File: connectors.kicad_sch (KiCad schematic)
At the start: 17 parts, among them J1 USB_C_Receptacle_USB2.0, J2 Power_Input, J3 Conn_01x11_Socket, J4 MOTOR_1_OUTPUT, J5 MOTOR_2_OUTPUT, J6 MOTOR_3_OUTPUT, J7 MOTOR_4_OUTPUT, J8 Conn_01x03_Socket, J9 Conn_01x11_Socket, U3 USBLC6-2SC6

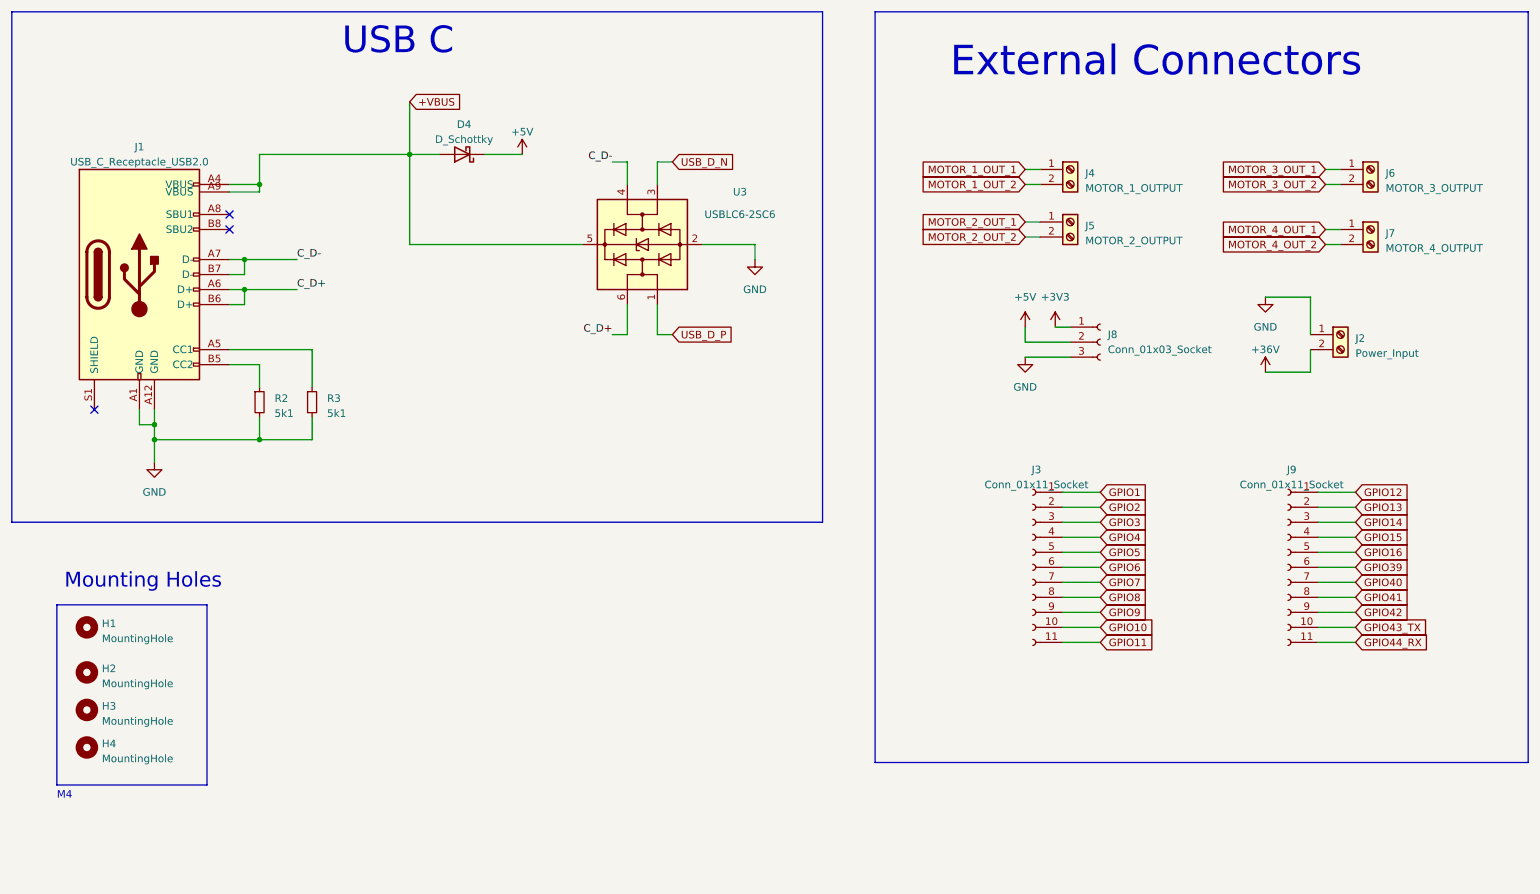
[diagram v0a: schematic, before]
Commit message: checkpoint for backup
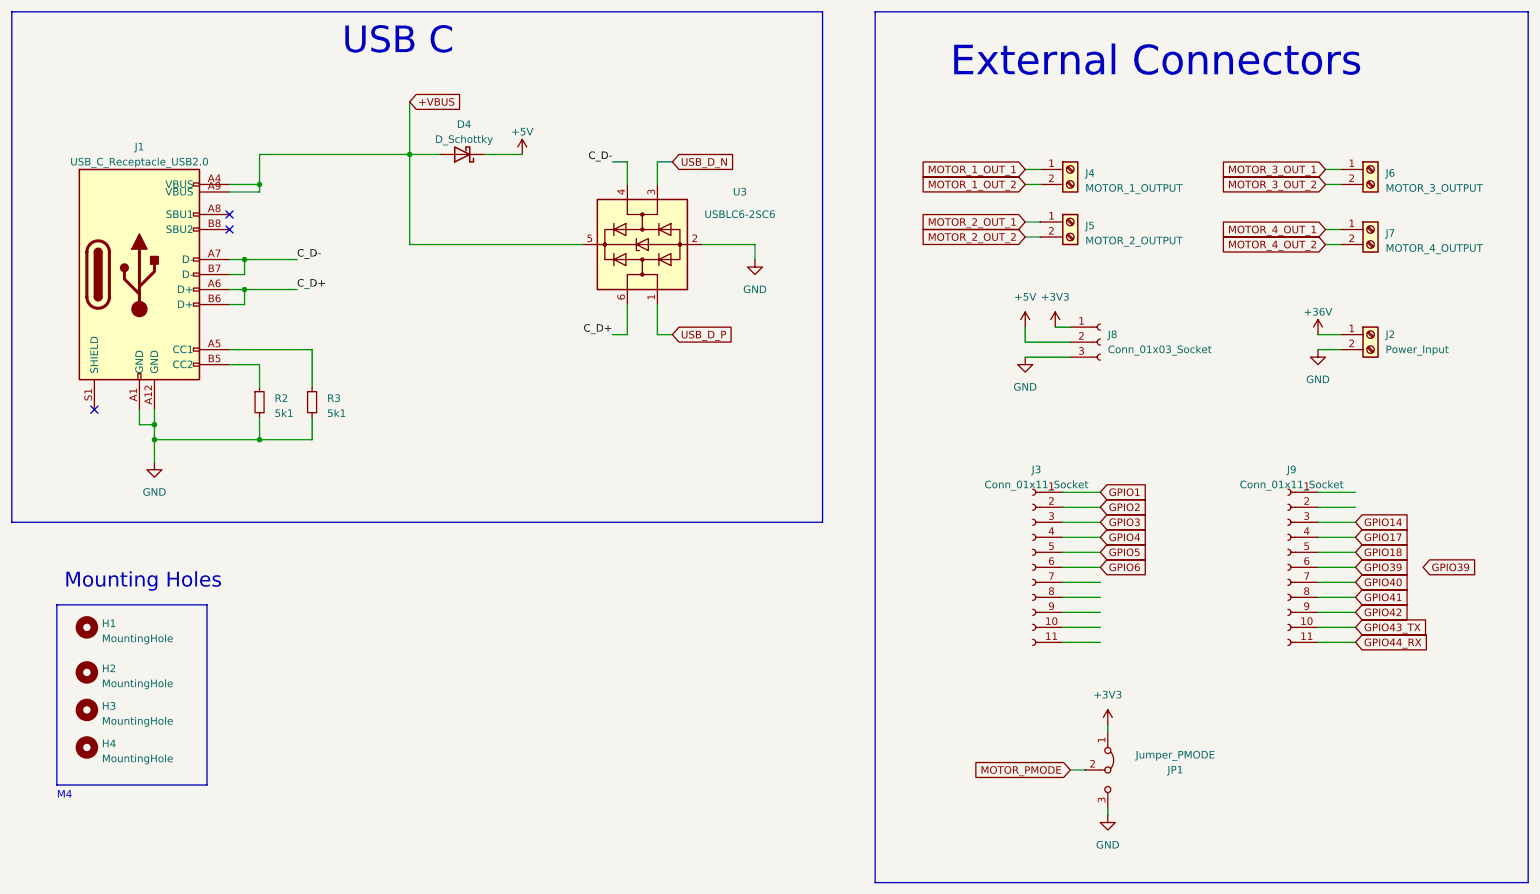
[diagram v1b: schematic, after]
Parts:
- added JP1: Jumper_PMODE, Connector_PinHeader_2.54mm:PinHeader_1x03_P2.54mm_Vertical_SMD_Pin1Right, symbol Jumper:Jumper_3_Bridged12
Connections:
- net +36V: now also J2.1 (Pin_1); no longer J2.2 (Pin_2)
- net +3V3: now also JP1.1 (A)
- net GND: now also J2.2 (Pin_2), JP1.3 (B); no longer J2.1 (Pin_1)
- net GPIO10: no longer names the net of J3.10 (Pin_10)
- net GPIO11: no longer names the net of J3.11 (Pin_11)
- net GPIO12: no longer names the net of J9.1 (Pin_1)
- net GPIO13: no longer names the net of J9.2 (Pin_2)
- net GPIO15 renamed GPIO17
- net GPIO16 renamed GPIO18
- net GPIO7: no longer names the net of J3.7 (Pin_7)
- net GPIO8: no longer names the net of J3.8 (Pin_8)
- net GPIO9: no longer names the net of J3.9 (Pin_9)
- new net MOTOR_PMODE: JP1.2 (C)
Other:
- moved on the sheet: J2
